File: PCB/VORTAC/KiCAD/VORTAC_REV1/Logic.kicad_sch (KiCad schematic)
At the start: 30 parts, among them U1 TLV73333PDBV, U3 EE-SX3350, U4 TPS54335ADRCR, U5 AS5047D, U7 EE-SX3350

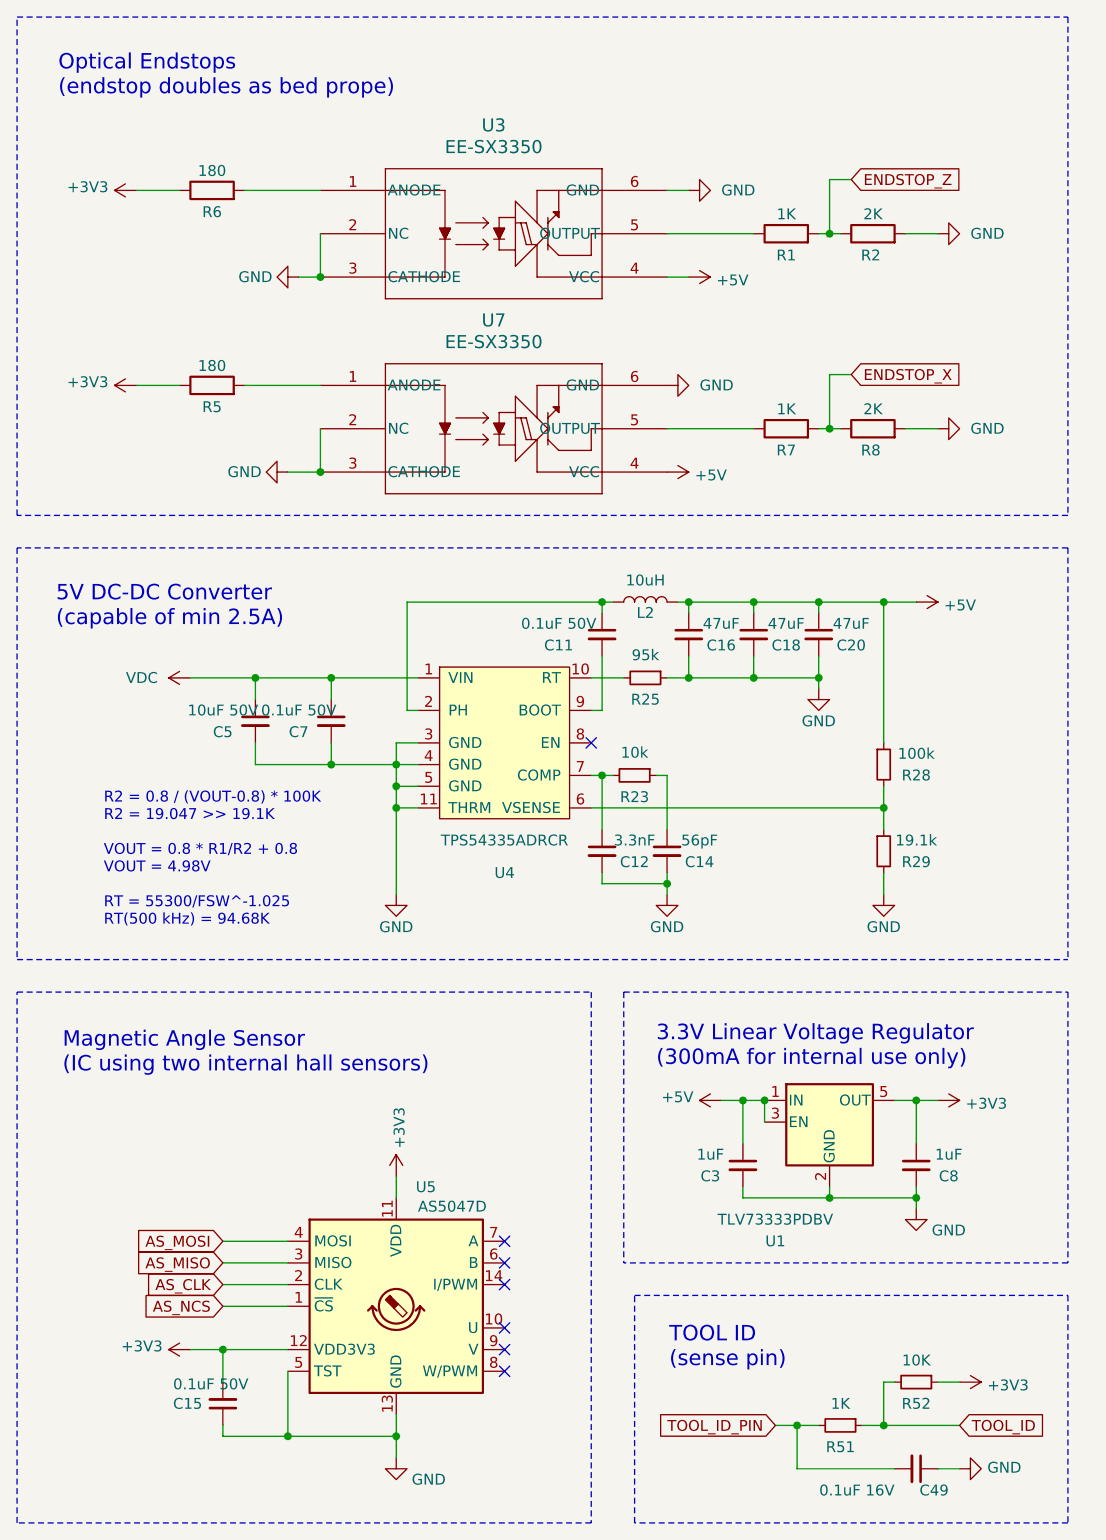
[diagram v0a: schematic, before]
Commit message: Gschenkle
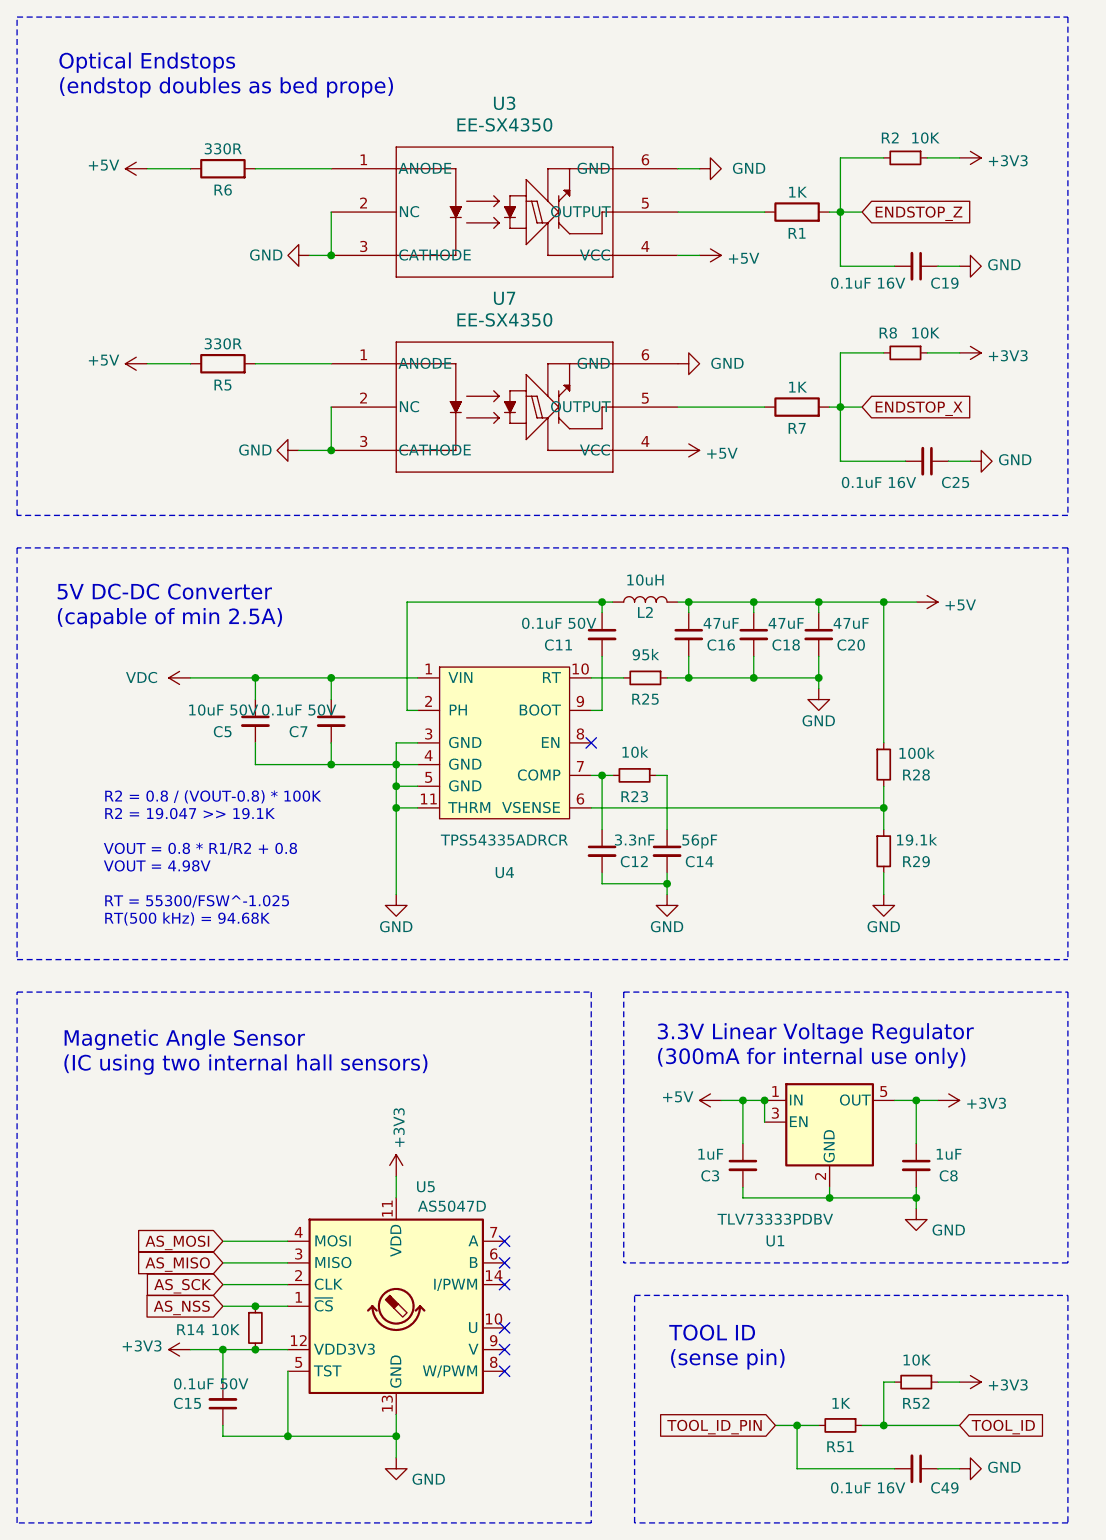
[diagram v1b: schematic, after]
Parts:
- removed R2, R8: 2K, Resistor_SMD:R_0603_1608Metric, symbol Device:R
- added C19, C25: 0.1uF 16V, Capacitor_SMD:C_0402_1005Metric, symbol Device:C_Small
- added R14, R2, R8: 10K, Resistor_SMD:R_0402_1005Metric, symbol Device:R_Small
- R5, R6: value 180 -> 330R
- U3, U7: value EE-SX3350 -> EE-SX4350; LCSC C7470740 -> C17524058
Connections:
- net +3V3: now also R14.2, R2.1, R8.1; no longer R5.1, R6.1
- net +5V: now also R5.1, R6.1
- net ENDSTOP_X: now also C25.2, R8.2
- net ENDSTOP_Z: now also C19.2, R2.2
- net GND: now also C19.1, C25.1
- net AS_CLK renamed AS_SCK
- net AS_NCS renamed AS_NSS
- net AS_NSS: now also R14.1
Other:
- moved on the sheet: R1, R5, R6, R7, U3, U7
